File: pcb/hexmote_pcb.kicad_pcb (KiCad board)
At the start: 2 copper layers, 90 x 40 mm, 22 parts, among them J2 LiPo Cell, J3 Conn_01x10_Pin, SW1 SW_Push_45deg, SW10 SW_SPDT, SW2 SW_Push_45deg, SW3 SW_Push_45deg, SW4 SW_Push_45deg, SW5 SW_Push_45deg, SW6 SW_Push_45deg, SW7 SW_Push_45deg, SW8 SW_Push_45deg, U1 SuperMini nRF52840, U2 Joystick

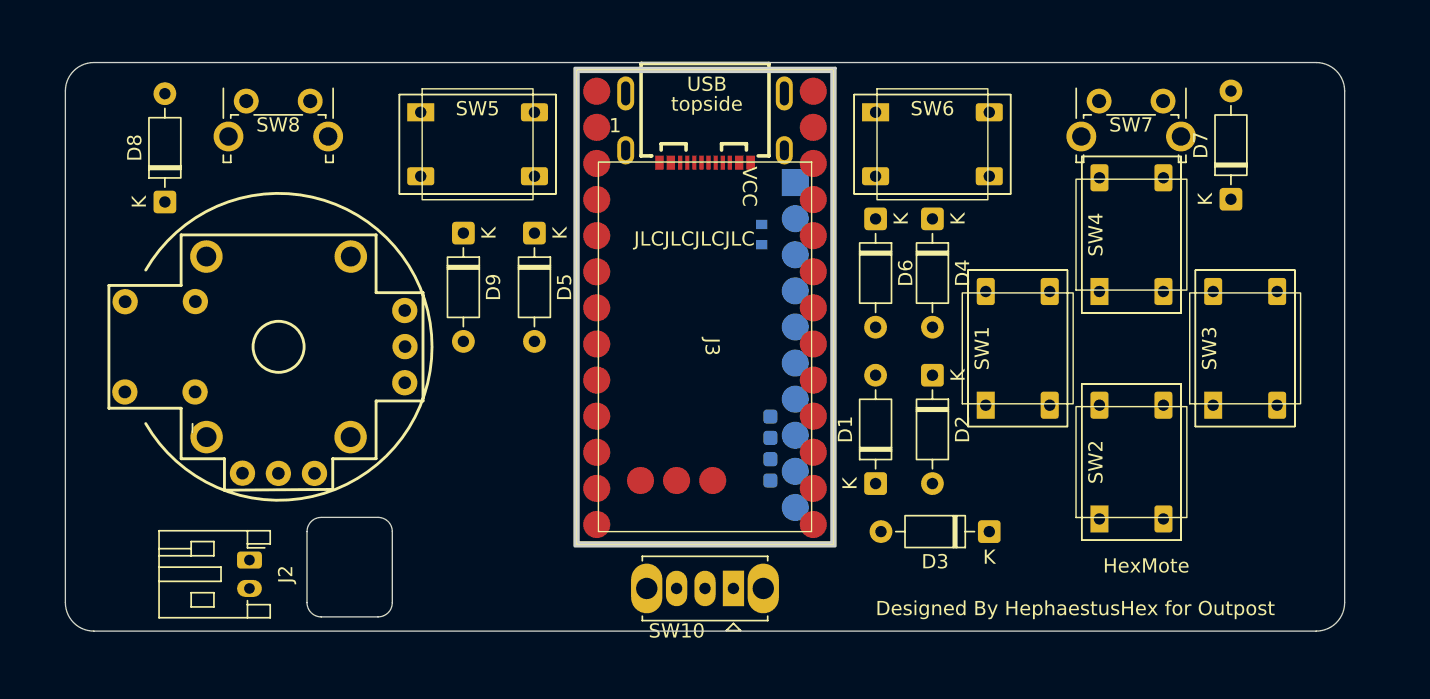
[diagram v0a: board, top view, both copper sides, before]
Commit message: finished PCB
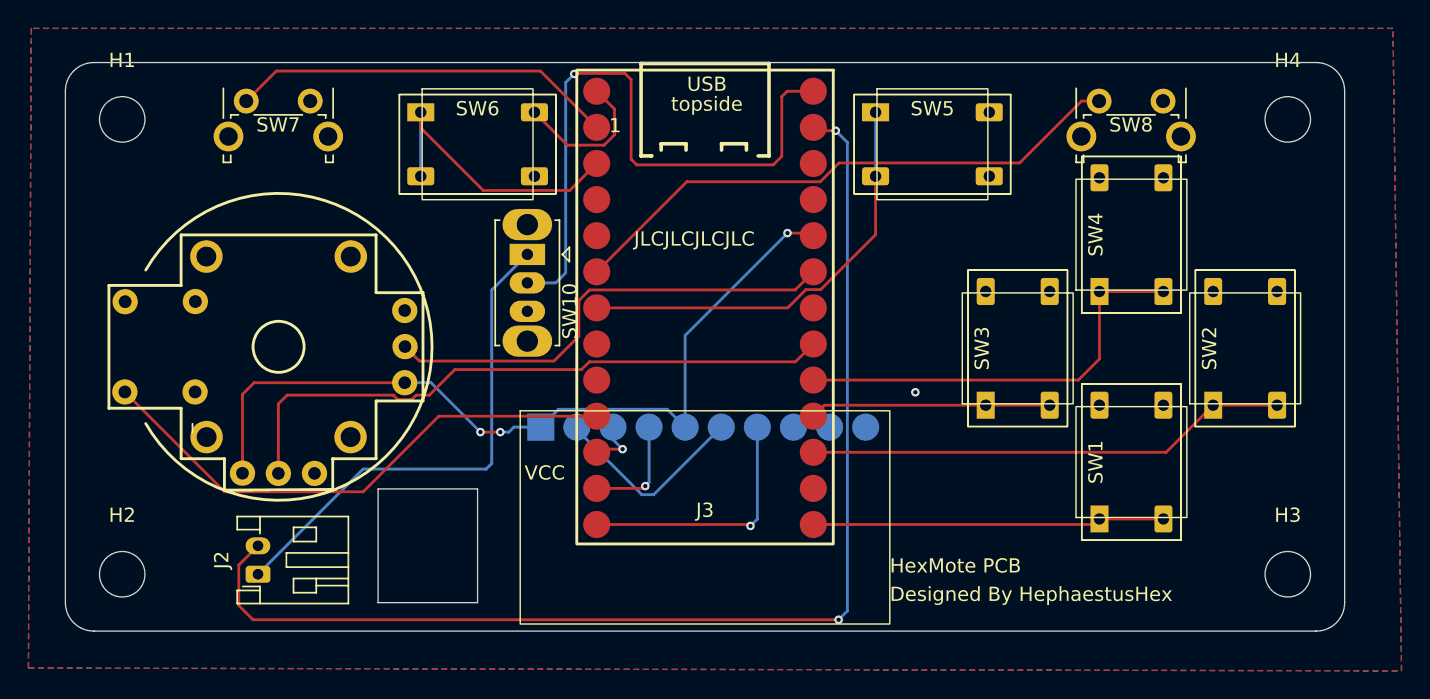
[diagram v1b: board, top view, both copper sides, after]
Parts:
- removed D1, D2, D3, D4, D5, D6, D7, D8, D9: 1N4148, Diode_THT:D_DO-35_SOD27_P7.62mm_Horizontal
- added H1: MountingHole, MountingHole:MountingHole_3.2mm_M3, F.Cu at (115.3, 81.4)
- added H2: MountingHole, MountingHole:MountingHole_3.2mm_M3, F.Cu at (115.3, 113.4)
- added H3: MountingHole, MountingHole:MountingHole_3.2mm_M3, F.Cu at (197.3, 113.4)
- added H4: MountingHole, MountingHole:MountingHole_3.2mm_M3, F.Cu at (197.3, 81.4)
- SW1, SW2, SW3, SW4, SW5, SW6, SW7, SW8: value SW_Push_45deg -> SW_Push
- moved SW7 60.0 mm to (124.1, 80.1)
- moved SW8 60.0 mm to (184.1, 80.1)
- moved SW5 32.0 mm to (172.3, 83.1)
- moved SW6 32.0 mm to (140.3, 83.1)
- moved SW10 27.6 mm to (143.8, 90.9), turned to -90 degrees
- moved SW3 16.0 mm to (178.3, 97.5)
- moved J3 12.0 mm to (156.3, 109.4), turned to 0 degrees
- moved SW1 11.3 mm to (186.3, 105.5)
- moved SW2 11.3 mm to (194.3, 97.5)
- moved J2 1.17 mm to (124.9, 113.4), turned to 90 degrees
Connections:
- SW1 pad 1: COL1 -> A
- SW1 pad 2: Net-(D1-A) -> GND
- SW2 pad 1: COL2 -> B
- SW2 pad 2: Net-(D2-A) -> GND
- SW3 pad 1: COL3 -> X
- SW3 pad 2: Net-(D3-A) -> GND
- SW4 pad 1: COL1 -> Y
- SW4 pad 2: Net-(D4-A) -> GND
- SW5 pad 1: COL2 -> +
- SW5 pad 2: Net-(D5-A) -> GND
- SW6 pad 1: COL3 -> -
- SW6 pad 2: Net-(D6-A) -> GND
- SW7 pad 1: COL1 -> L
- SW7 pad 2: Net-(D7-A) -> GND
- SW8 pad 1: COL2 -> R
- SW8 pad 2: Net-(D8-A) -> GND
- U1 pad 1: unconnected-(U1-P0.06-Pad1) -> L
- U1 pad 10: COL3 -> SCL
- U1 pad 11: unconnected-(U1-P1.04-LF-Pad11) -> SDA
- U1 pad 12: unconnected-(U1-P1.06-LF-Pad12) -> INT
- U1 pad 17: unconnected-(U1-P0.31-LF-Pad17) -> VRx
- U1 pad 18: VRy -> unconnected-(U1-P0.29-LF-Pad18)
- U1 pad 19: VRx -> VRy
- U1 pad 2: unconnected-(U1-P0.08-Pad2) -> -
- U1 pad 20: SCL -> Y
- U1 pad 21: SDA -> X
- U1 pad 22: INT -> B
- U1 pad 24: unconnected-(U1-P0.09-LF-Pad24) -> A
- U1 pad 5: ROW1 -> R
- U1 pad 6: ROW2 -> +
- U1 pad 7: ROW3 -> unconnected-(U1-P0.22-Pad7)
- U1 pad 8: COL1 -> unconnected-(U1-P0.24-Pad8)
- U1 pad 9: COL2 -> SEL
- U2 pad B1A: COL3 -> SEL
- U2 pad B2A: SEL- -> GND
- U2 pad H1: +3.3V -> +3V3
- U2 pad V1: +3.3V -> +3V3
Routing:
- net Net-(J2-Pin_2): track 0.00 -> 84.0 mm, vias 0 -> 2
- net +3V3: track 0.00 -> 58.2 mm, vias 0 -> 3
- net VRy: track 0.00 -> 44.8 mm
- net Net-(SW10-B): track 0.00 -> 44.6 mm, vias 0 -> 1
- net R: track 0.00 -> 40.3 mm
- net SEL: track 0.00 -> 38.3 mm
- net Net-(J2-Pin_1): track 0.00 -> 35.4 mm
- net B: track 0.00 -> 34.0 mm
- net VRx: track 0.00 -> 33.2 mm
- net +: track 0.00 -> 30.4 mm
- net Y: track 0.00 -> 30.0 mm
- net L: track 0.00 -> 27.2 mm
- net A: track 0.00 -> 24.8 mm
- net GND: track 0.00 -> 24.7 mm
- net -: track 0.00 -> 20.6 mm
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- added copper zone on B.Cu, net GND
- added copper zone on F.Cu, net GND
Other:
- outline, holes or cut-outs redrawn
- board text added: "Designed By HephaestusHex"
- board text added: "HexMote PCB"
- board text removed: "Designed By HephaestusHex for Outpost"
- board text removed: "HexMote"
